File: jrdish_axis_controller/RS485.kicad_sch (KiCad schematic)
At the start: 0 parts

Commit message: Updates
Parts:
- added C21, C26: 100nF, PCM_JLCPCB:C_0402, symbol PCM_JLCPCB-Capacitors:0402,100nF
- added C22, C27: 10uF, PCM_JLCPCB:C_0402, symbol PCM_JLCPCB-Capacitors:0402,10uF
- added C23, C25, C28, C30, C31: 10nF, PCM_JLCPCB:C_0402, symbol PCM_JLCPCB-Capacitors:0402,10nF
- added C24, C29: 1uF, PCM_JLCPCB:C_0402, symbol PCM_JLCPCB-Capacitors:0402,1uF
- added CN3: KF2EDGR-2.54-4P, MyParts:CONN-TH_4P-P2.54_KF2EDGR-2.54-4P, symbol MyParts:KF2EDGR-2.54-4P
- added H3: 210S-1*2P L=11.6MMGold-plated black, MyParts:HDR-TH_2P-P2.54-V-M-1, symbol MyParts:210S-1*2PL=11.6MMGold-platedblack
- added L1, L2, L3, L4: BLM15EX331SN1D, MyParts:L0402, symbol MyParts:BLM15EX331SN1D
- added R15: 4.7kΩ, PCM_JLCPCB:R_0402, symbol PCM_JLCPCB-Resistors:0402,4.7kΩ
- added R16: 120Ω, PCM_JLCPCB:R_0805, symbol PCM_JLCPCB-Resistors:0805,120Ω
- added U2: ISOW1432BDFMR, MyParts:SOIC-20_L12.8-W7.5-P1.27-LS10.3-BL, symbol MyParts:ISOW1432BDFMR
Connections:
- new net: C23.1, C24.1, C25.1, L2.2, U2.9 (VDD)
- new net: C28.1, C29.1, C30.1, L3.1, U2.12 (VISOOUT), U2.13 (MODE)
- new net: C28.2, C29.2, C30.2, L4.1, U2.11 (GND2)
- new net: C21.1, C22.1, L1.2, R15.1, U2.1 (VIO)
- new net: H3.2, R16.2
- new net: C26.1, C27.1, L3.2, U2.16 (VISOIN)
- new net: R15.2, U2.8 (EN/FLT)
- new net 3.3V: L1.1, L2.1
- new net GND: C21.2, C22.2, C23.2, C24.2, C25.2, U2.10 (GND1), U2.6 (GNDIO)
- new net GND_RS485: C26.2, C27.2, C31.1, CN3.3, L4.2, U2.15 (GISOIN)
- new net RS485_CHASSIS: C31.2, CN3.4
- new net RS485_DE_MCU: U2.3 (DE), U2.5 (~{RE})
- new net RS485_RX: CN3.1, R16.1, U2.18 (Z), U2.19 (B)
- new net RS485_TX: CN3.2, H3.1, U2.17 (Y), U2.20 (A)
- new net USART1_RX_MCU: U2.4 (R)
- new net USART1_TX_MCU: U2.2 (D)
- no-connect marks 0 -> 2
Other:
- note added: "C23 and C28 need to be 1mm from their respecive pins."
- note added: "Caps near VIO"
- note added: "HF Noise Bleed"
- note added: "Isolated RS485"
- note added: "L1/L2/L3/L4 are 205mΩ 330Ω@100MHz 700mA ±25% 0402 Ferrite Beads"
- note added: "Note: RS485 Cable Shield connects to Earth gound at the host"
- note added: "RS485_CHASSIS connects directly to chassis"

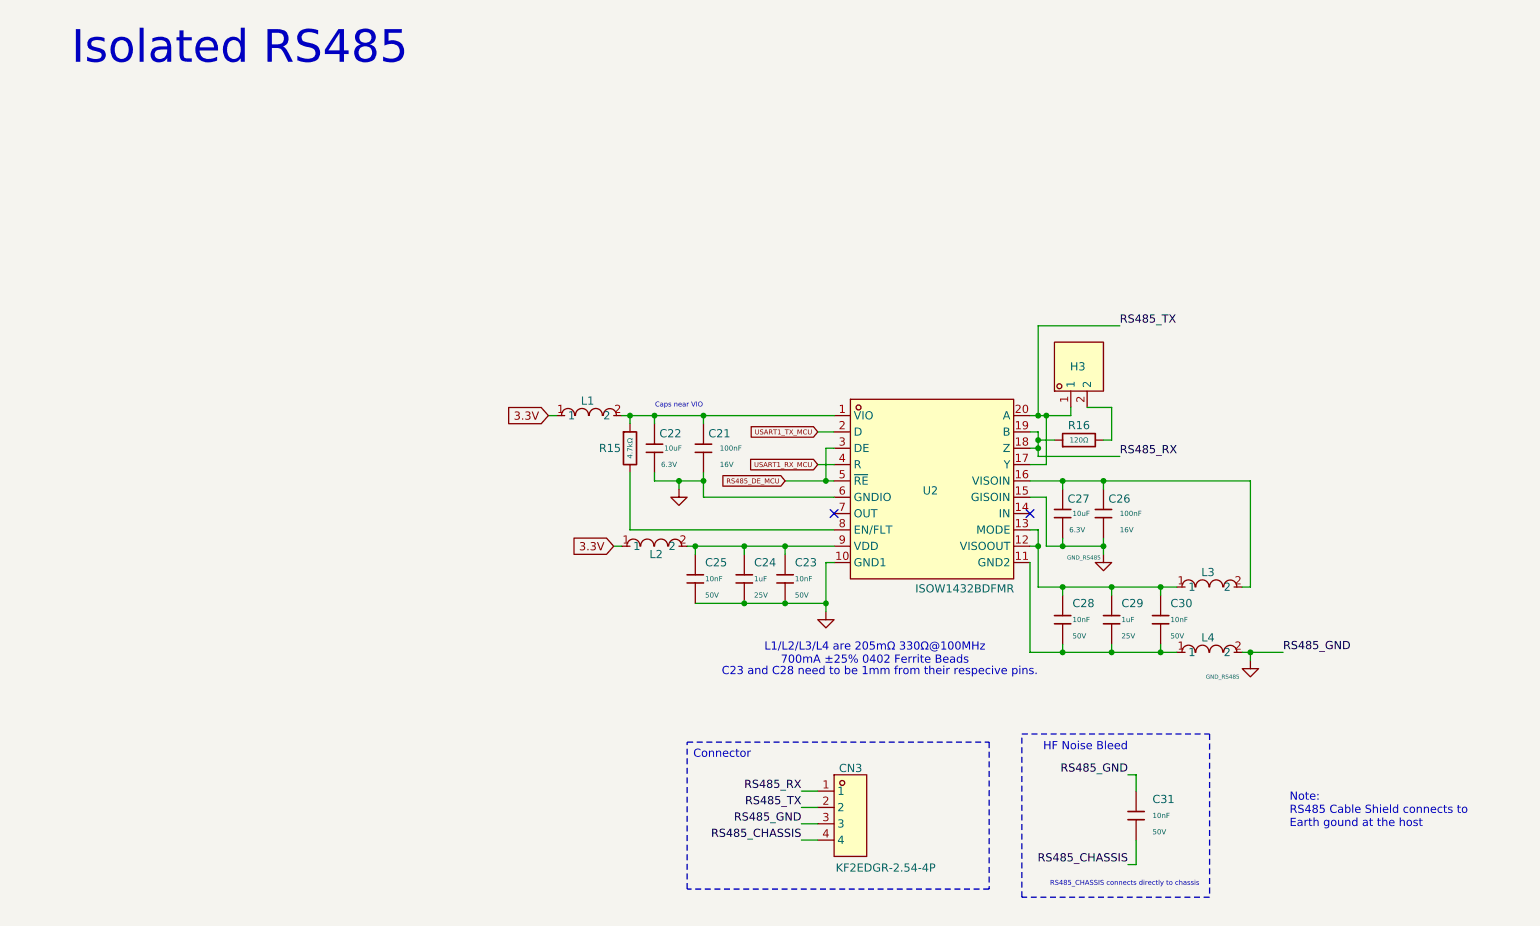
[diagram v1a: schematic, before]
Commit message: Passes ERC
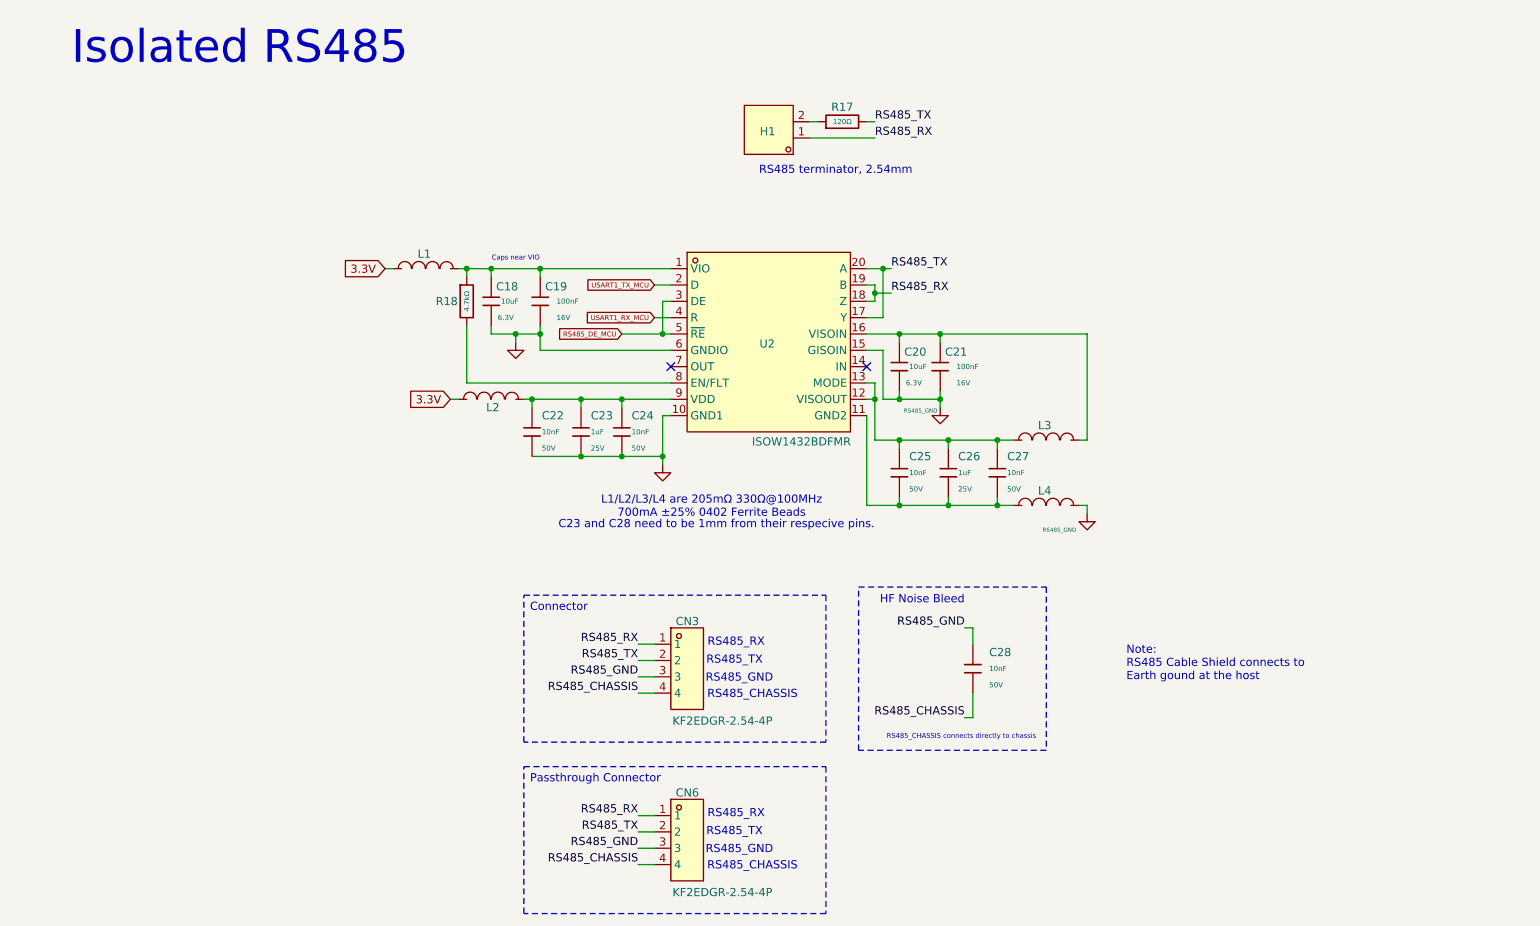
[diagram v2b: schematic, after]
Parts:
- added CN6: KF2EDGR-2.54-4P, MyParts:CONN-TH_4P-P2.54_KF2EDGR-2.54-4P, symbol MyParts:KF2EDGR-2.54-4P
- renumbered C22 to C18, C21 to C19, C27 to C20, C26 to C21, C25 to C22, C24 to C23, C23 to C24, C28 to C25, C29 to C26, C30 to C27, C31 to C28, H3 to H1, R16 to R17, R15 to R18
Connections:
- net RS485_CHASSIS: now also CN6.4
- net RS485_RX: now also H1.1, CN6.1; no longer R17.1
- net RS485_TX: now also R17.2, CN6.2; no longer H1.1
- net at H1.2: now also R17.1; no longer R17.2
- net GND_RS485 renamed RS485_GND
- net RS485_GND: now also CN6.3
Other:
- note added: "RS485 terminator, 2.54mm"
- note added: "RS485_CHASSIS"
- note added: "RS485_GND"
- note added: "RS485_RX"
- note added: "RS485_TX"
- moved on the sheet: C18, C19, C20, C21, C22, C23, C24, C25, C26, C27, C28, CN3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
